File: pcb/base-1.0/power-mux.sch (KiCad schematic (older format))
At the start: 23 parts, among them Q201 IRF7324TRPBF, Q202 IRF7324TRPBF, Q203 IRF7324TRPBF, U201 LTC4417

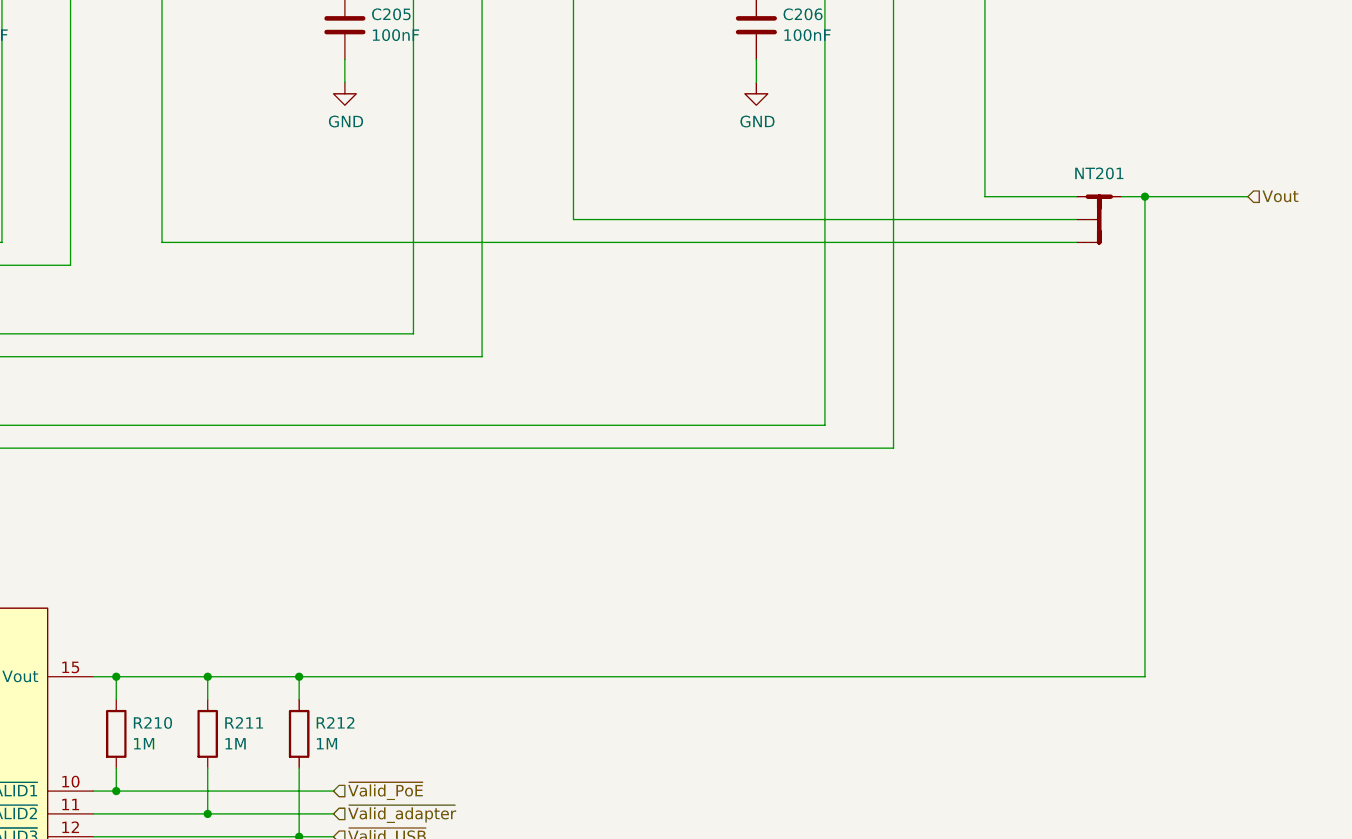
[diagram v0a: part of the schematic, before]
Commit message: o Much more PCB work.
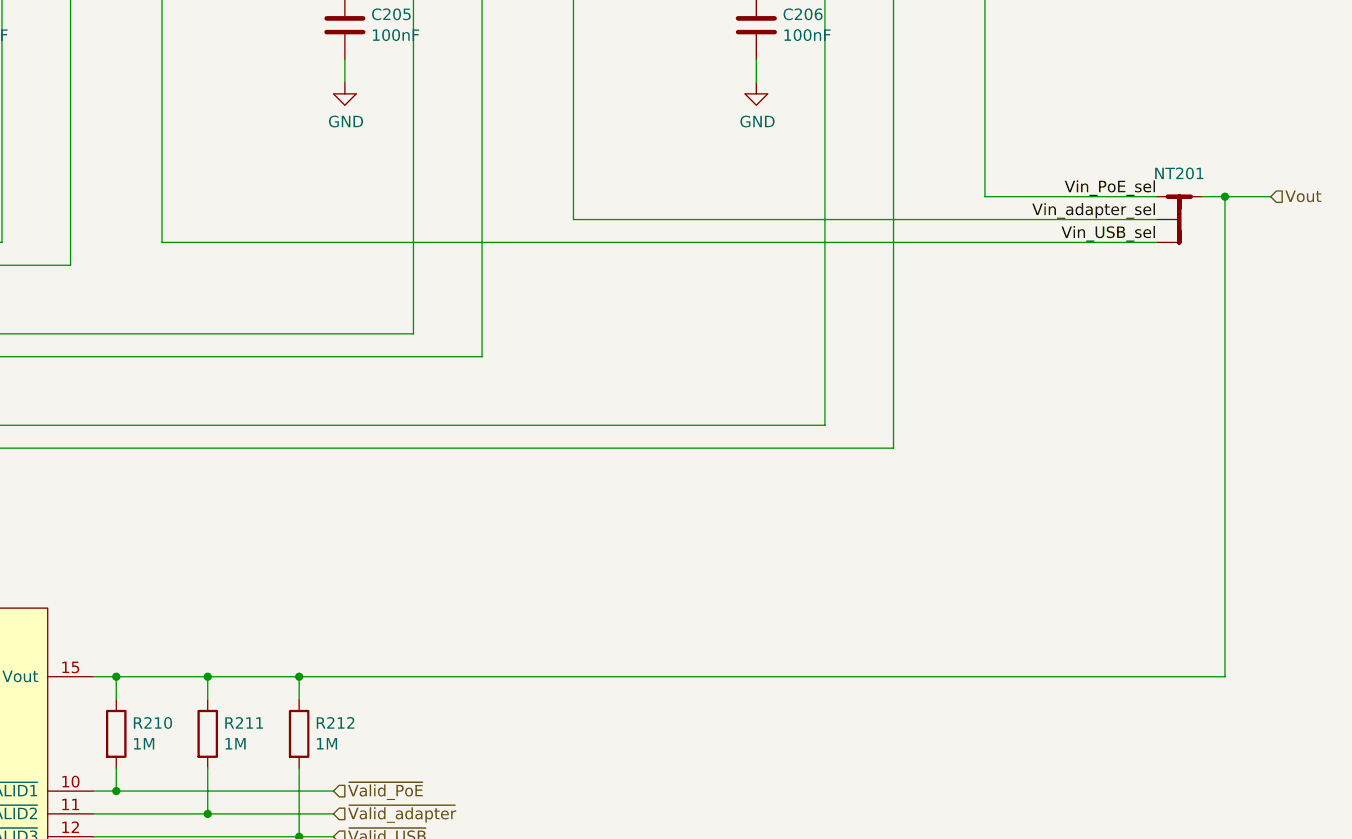
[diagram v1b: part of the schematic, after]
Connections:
- net Vin_PoE_sel: now reaches NT201.1, Q203.5 (D), Q203.6 (D)
- net Vin_adapter_sel: now reaches NT201.2, Q202.5 (D), Q202.6 (D)
- net Vin_USB_sel: now reaches NT201.3, Q201.5 (D), Q201.6 (D)
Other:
- moved on the sheet: NT201
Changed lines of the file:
@@
 TODO:\n* Select MOSFETs. One option: CSD75207W15\n* Calculate resistor values
 Wire Wire Line
-	6500 5500 10200 5500
+	6500 5500 10550 5500
 Connection ~ 5900 1900
 Wire Wire Line
@@
 	9300 1800 9500 1800
 Wire Wire Line
-	9500 3400 9900 3400
+	9500 3400 10250 3400
 Wire Wire Line
 	9500 1900 9500 3400
@@
 Text HLabel 1100 800  0    50   Input ~ 0
 Vin_PoE
-Text HLabel 10650 3400 2    50   Input ~ 0
+Text HLabel 10750 3400 2    50   Input ~ 0
 Vout
 Wire Wire Line
-	10200 3400 10650 3400
-Connection ~ 10200 3400
-Wire Wire Line
-	10100 3400 10200 3400
+	10550 3400 10750 3400
+Connection ~ 10550 3400
+Wire Wire Line
+	10450 3400 10550 3400
 $Comp
 L unlockoslo:Net-Tie_3_to_1 NT201
 U 1 1 5D02029B
-P 10000 3400
-F 0 "NT201" H 10000 3500 50  0000 C CNN
-F 1 "Net-Tie_3_to_1" H 10000 3490 50  0001 C CNN
-F 2 "NetTie:NetTie-4_SMD_Pad0.5mm" H 10000 3400 50  0001 C CNN
-F 3 "~" H 10000 3400 50  0001 C CNN
-	1    10000 3400
-	1    0    0    -1
-$EndComp
-Wire Wire Line
-	10200 5500 10200 3400
+P 10350 3400
+F 0 "NT201" H 10350 3500 50  0000 C CNN
+F 1 "Net-Tie_3_to_1" H 10350 3490 50  0001 C CNN
+F 2 "NetTie:NetTie-4_SMD_Pad0.5mm" H 10350 3400 50  0001 C CNN
+F 3 "~" H 10350 3400 50  0001 C CNN
+	1    10350 3400
+	1    0    0    -1
+$EndComp
+Wire Wire Line
+	10550 5500 10550 3400
 Connection ~ 1400 2200
 Wire Wire Line
@@
 	4600 5000 4600 4100
 Wire Wire Line
-	7700 3500 9900 3500
-Wire Wire Line
-	5900 3600 9900 3600
+	7700 3500 10250 3500
+Wire Wire Line
+	5900 3600 10250 3600
 Wire Wire Line
 	7700 1900 7700 3500
@@
 Wire Wire Line
 	5100 1900 5200 1900
+Text Label 10250 3600 2    50   ~ 0
+Vin_USB_sel
+Text Label 10250 3500 2    50   ~ 0
+Vin_adapter_sel
+Text Label 10250 3400 2    50   ~ 0
+Vin_PoE_sel
 $EndSCHEMATC

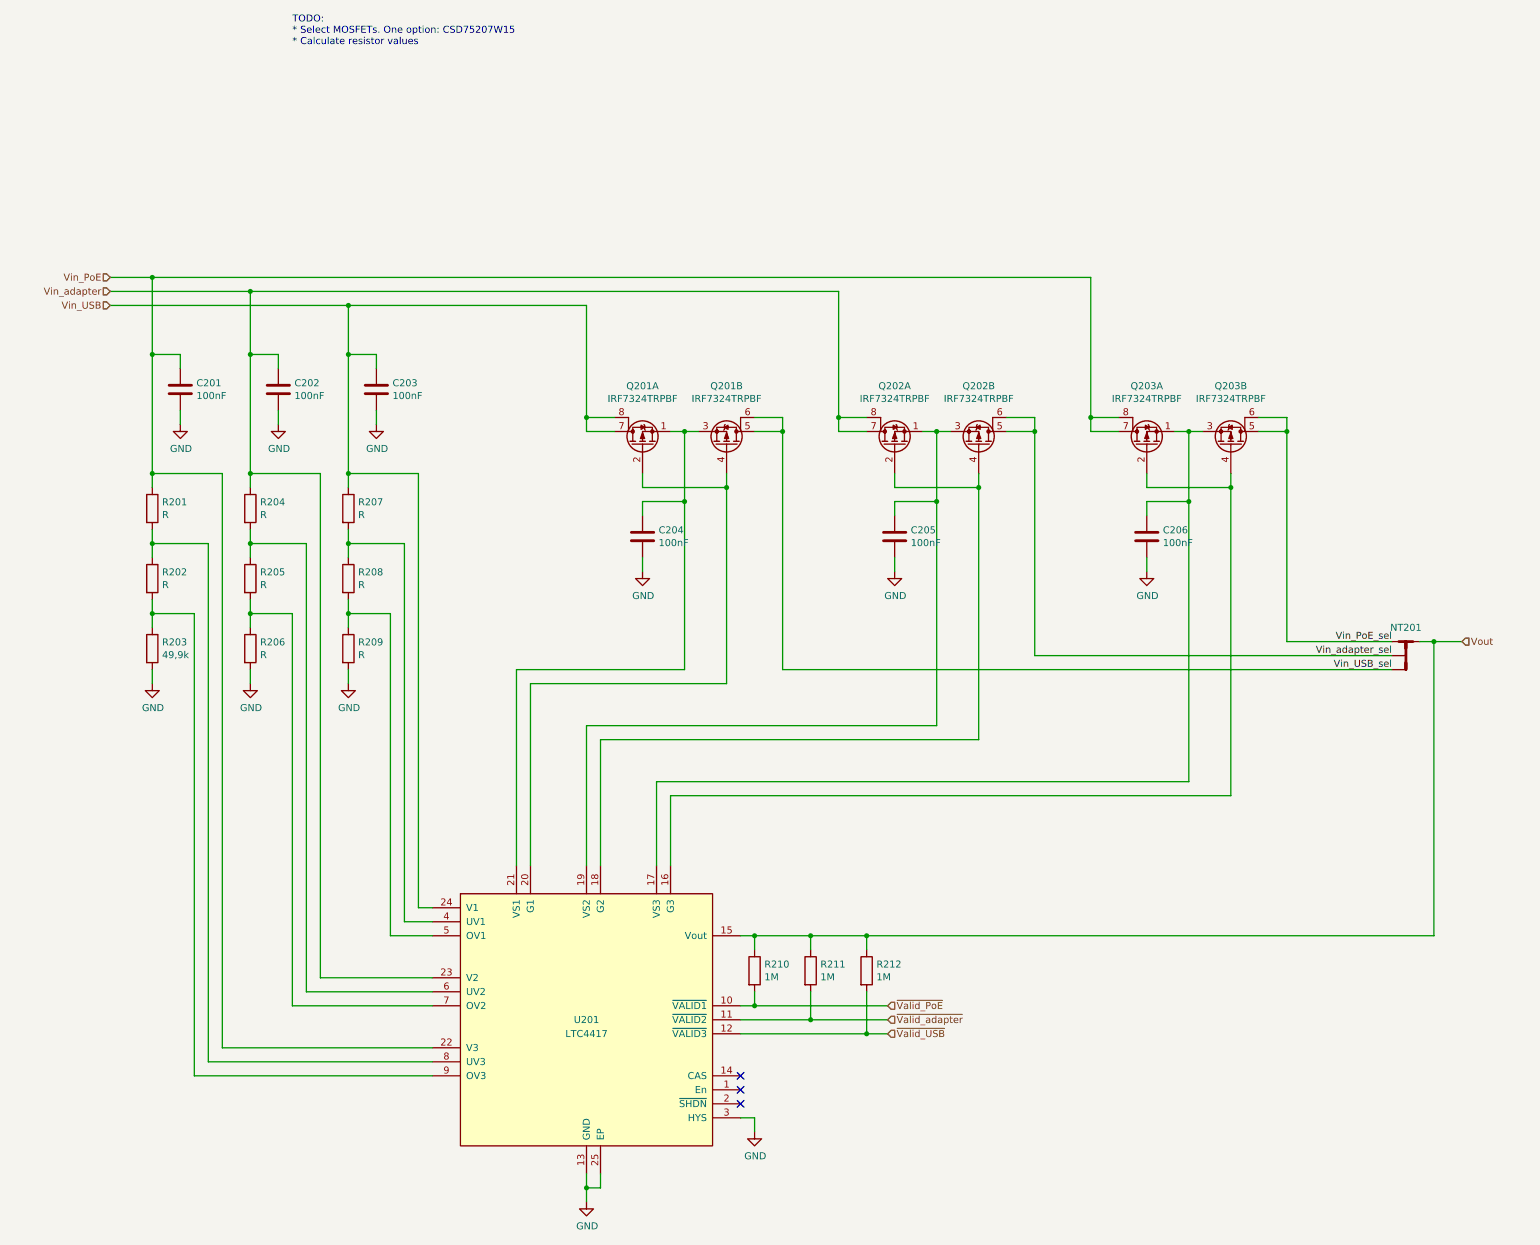
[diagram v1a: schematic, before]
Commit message: o More PCB work.
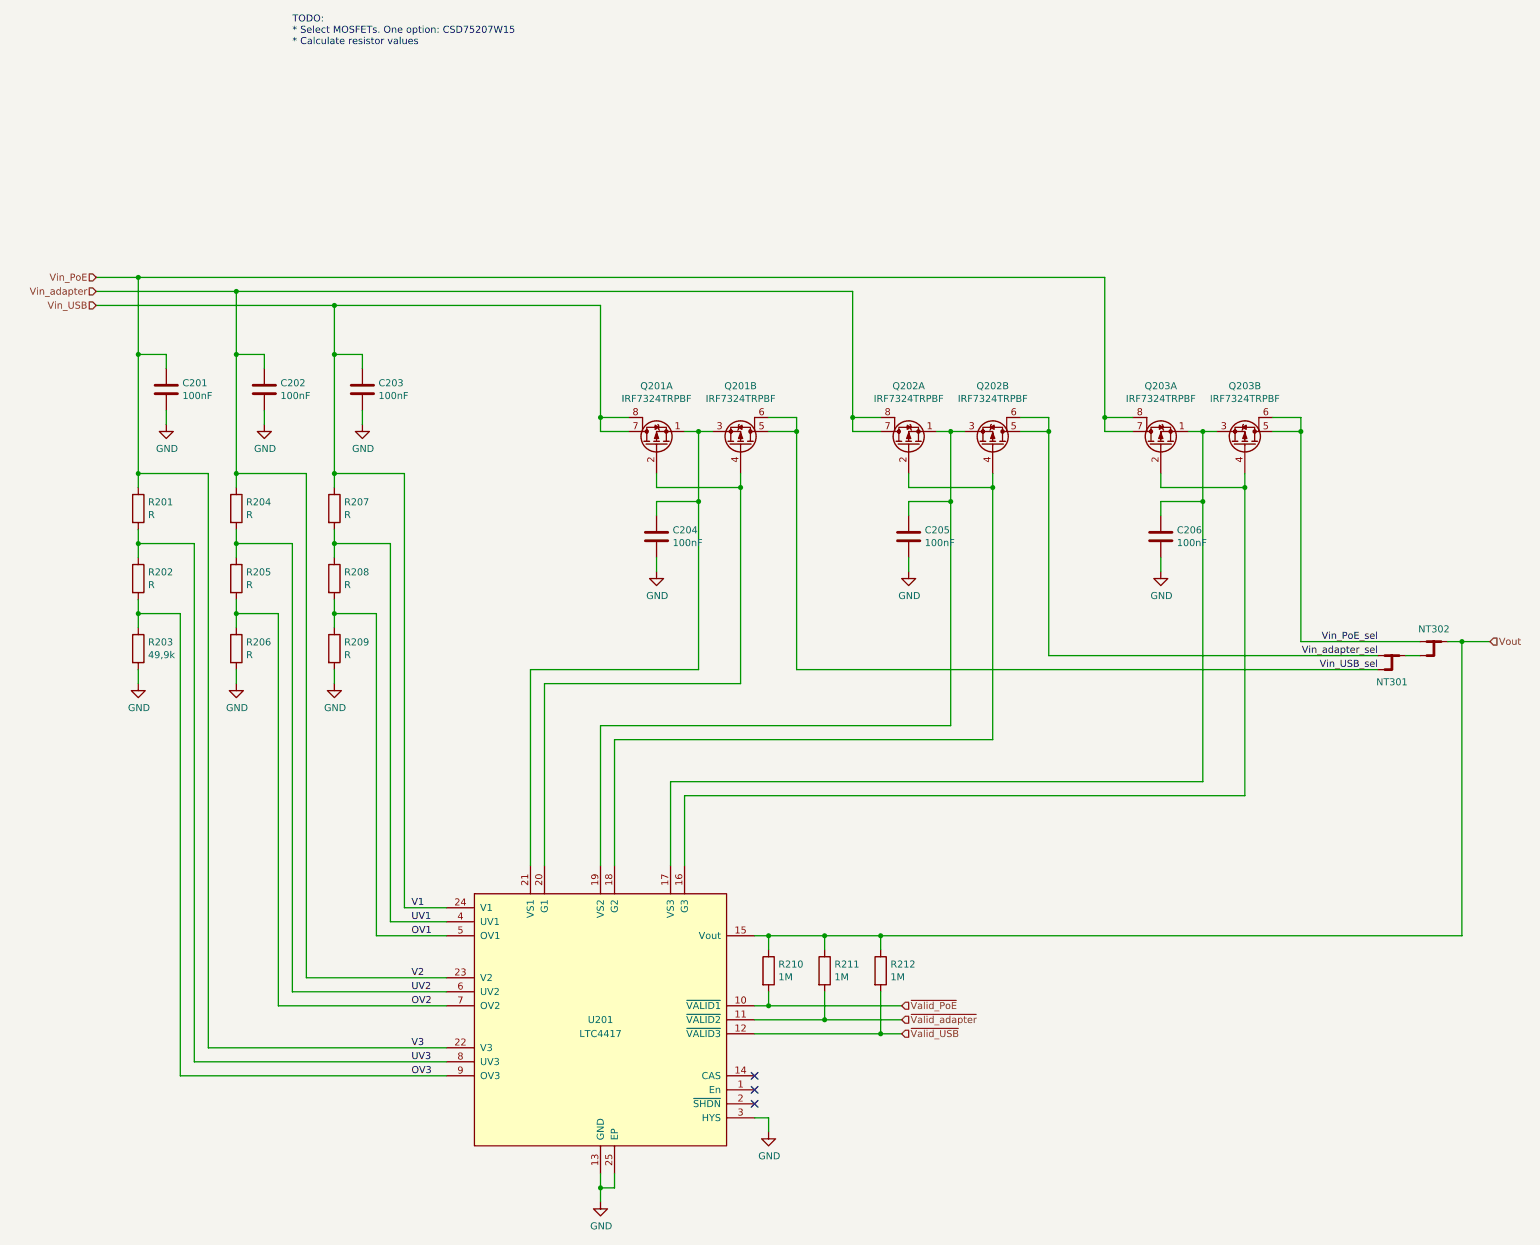
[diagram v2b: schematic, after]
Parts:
- removed NT201: Net-Tie_3_to_1, NetTie:NetTie-4_SMD_Pad0.5mm, symbol unlockoslo:Net-Tie_3_to_1
- added NT301, NT302: Net-Tie_3, UnlockOslo:NetTie-3_SMD_Pad0.5mm_132, symbol Device:Net-Tie_3
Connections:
- net Vin_PoE_sel: now also NT302.1
- net Vin_USB_sel: now also NT301.3
- net Vin_adapter_sel: now also NT301.1
- net Vout: now also NT302.2
- net UV3: now reaches R201.2, R202.1, U201.8 (UV3)
- net OV3: now reaches R202.2, R203.1, U201.9 (OV3)
- net UV2: now reaches R204.2, R205.1, U201.6 (UV2)
- net OV2: now reaches R205.2, R206.1, U201.7 (OV2)
- net UV1: now reaches R207.2, R208.1, U201.4 (UV1)
- net OV1: now reaches R208.2, R209.1, U201.5 (OV1)
- new net: NT301.2, NT302.3
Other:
- moved on the sheet: C201, C202, C203, C204, C205, C206, Q201A, Q201B, Q202A, Q202B, Q203A, Q203B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

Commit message: o 4 layers.
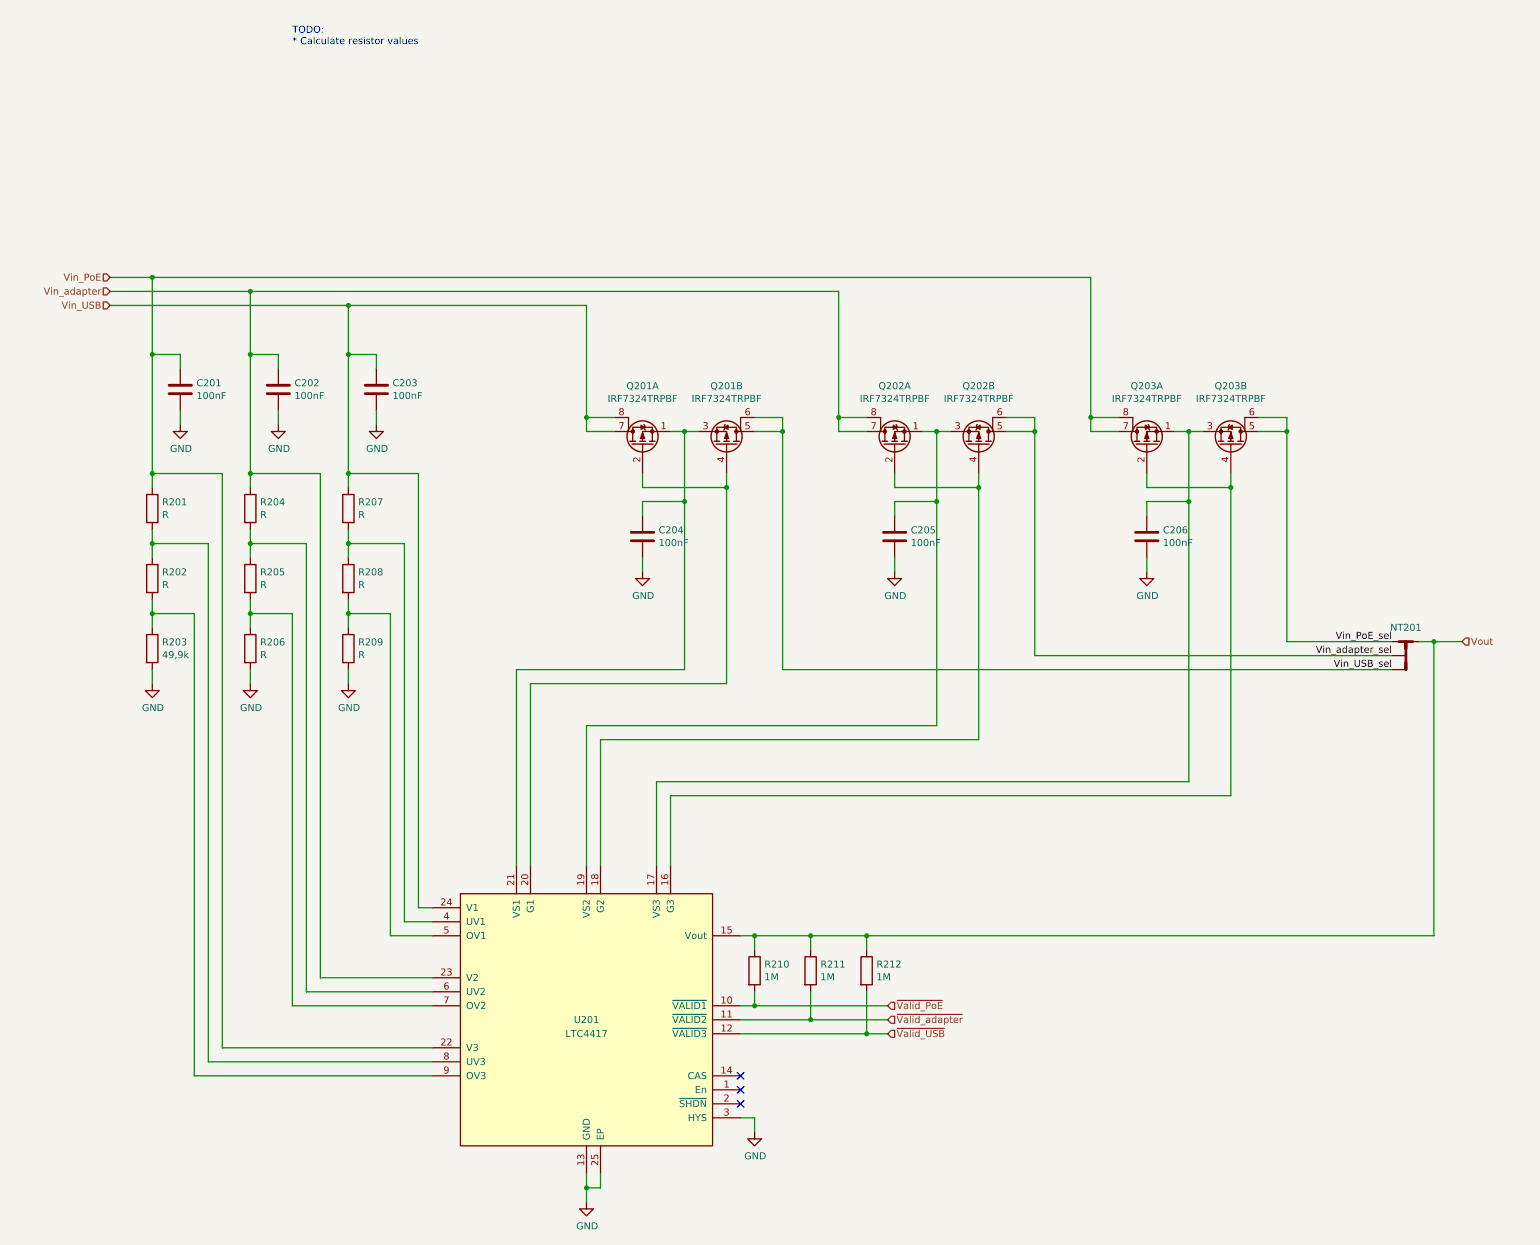
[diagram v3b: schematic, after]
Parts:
- removed NT301, NT302: Net-Tie_3, UnlockOslo:NetTie-3_SMD_Pad0.5mm_132, symbol Device:Net-Tie_3
- added NT201: Net-Tie_3_to_1, NetTie:NetTie-4_SMD_Pad0.5mm, symbol unlockoslo:Net-Tie_3_to_1
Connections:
- net Vin_PoE_sel: now also NT201.1
- net Vin_USB_sel: now also NT201.3
- net Vin_adapter_sel: now also NT201.2
- net Vout: now also NT201.4
- net OV1: no longer names the net of R208.2, R209.1, U201.5 (OV1)
- net OV2: no longer names the net of R205.2, R206.1, U201.7 (OV2)
- net OV3: no longer names the net of R202.2, R203.1, U201.9 (OV3)
- net UV1: no longer names the net of R207.2, R208.1, U201.4 (UV1)
- net UV2: no longer names the net of R204.2, R205.1, U201.6 (UV2)
- net UV3: no longer names the net of R201.2, R202.1, U201.8 (UV3)
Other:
- note added: "TODO:\n* Calculate resistor values"
- note removed: "TODO:\n* Select MOSFETs. One option: CSD75207W15\n* Calculate resistor values"
- moved on the sheet: C201, C202, C203, C204, C205, C206, Q201A, Q201B, Q202A, Q202B, Q203A, Q203B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
